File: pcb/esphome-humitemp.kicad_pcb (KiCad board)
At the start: 2 copper layers, 45 x 30 mm, 17 parts, among them J2 USB_IN, SW1 RESET, U1 SHT3x, U3 AMS1117-3.3, U4 ESP32-C3-MINI-1

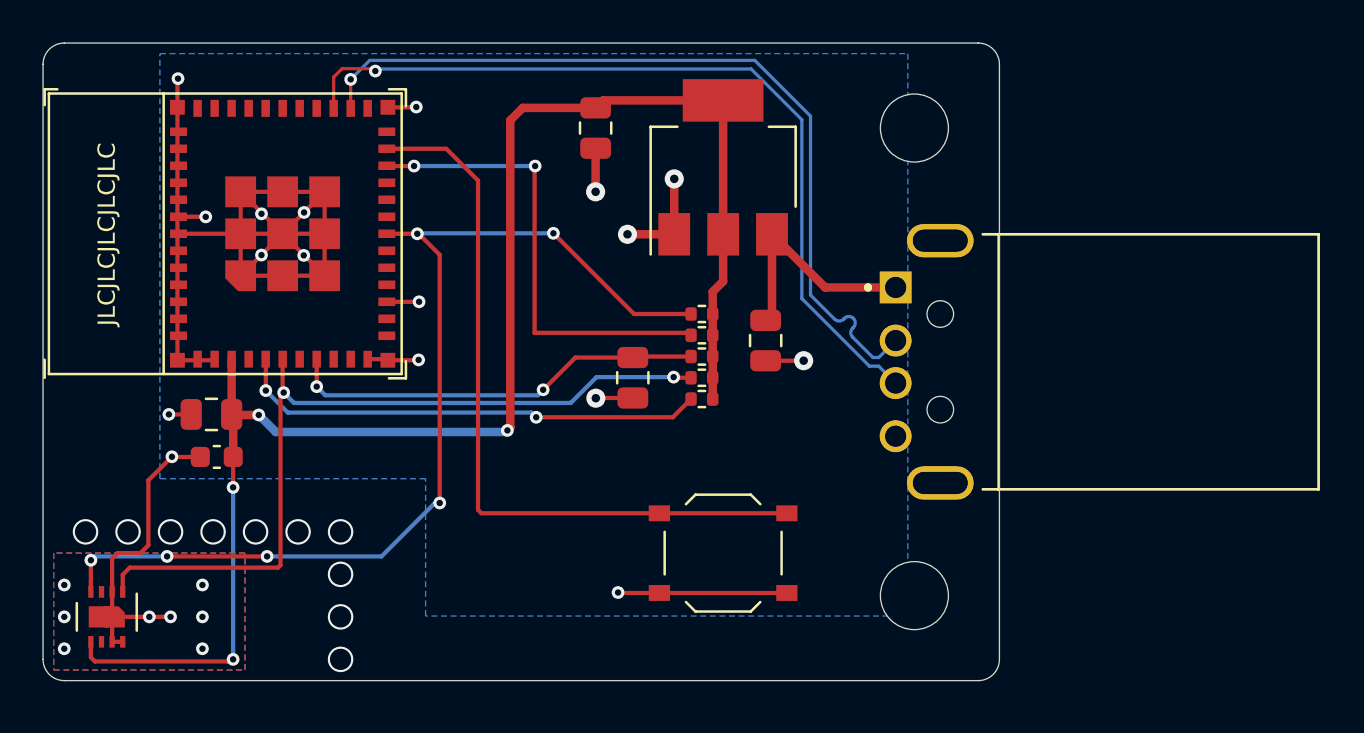
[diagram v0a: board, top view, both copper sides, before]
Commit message: rotate and send it
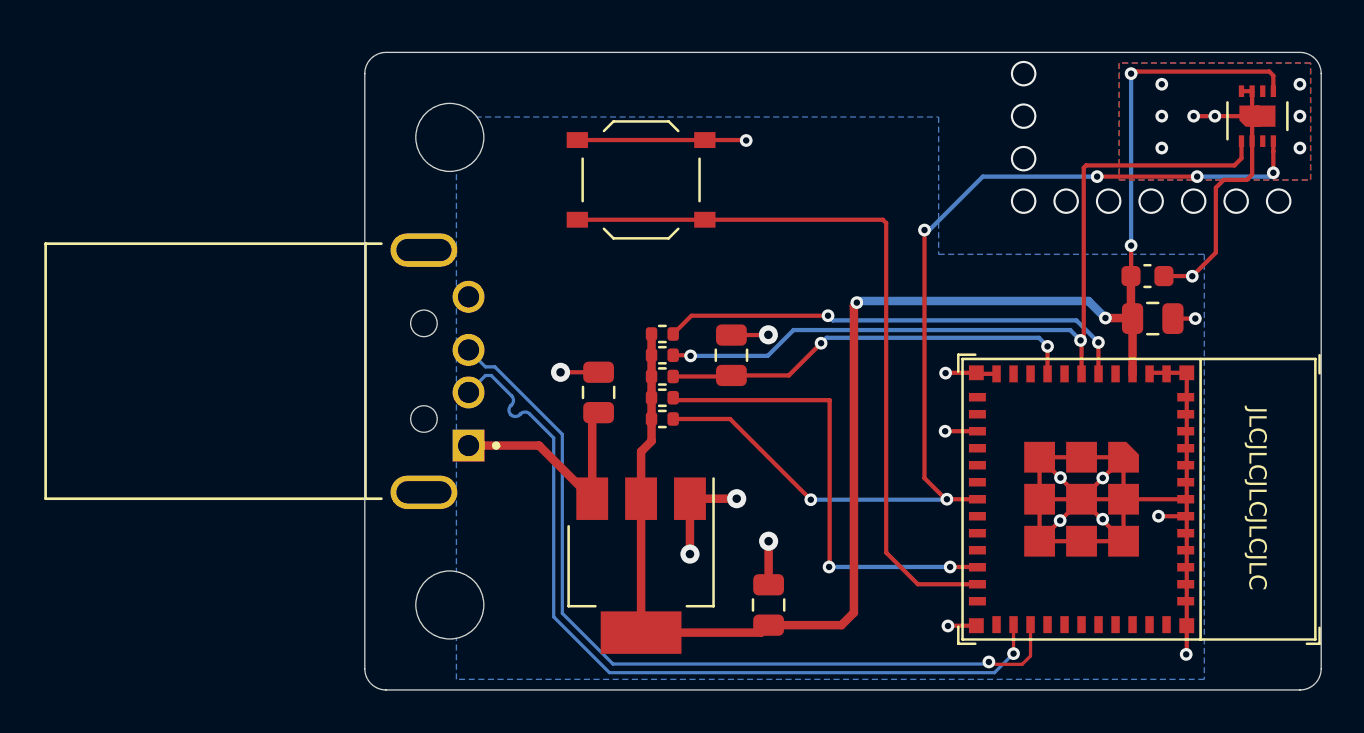
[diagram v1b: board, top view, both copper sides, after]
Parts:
- moved U1 59.0 mm to (147.1, 53.4), turned to 90 degrees
- moved U4 44.8 mm to (141.6, 71.5), turned to -90 degrees
- moved C5 44.6 mm to (142.0, 61.0), turned to 180 degrees
- moved C6 44.5 mm to (142.2, 63.0), turned to 180 degrees
- moved H1 31.3 mm to (109.1, 76.4), turned to 180 degrees
- moved H2 30.7 mm to (109.1, 54.4), turned to 180 degrees
- moved J2 24.3 mm to (107.9, 65.4), turned to -90 degrees
- moved C2 23.9 mm to (124.1, 76.4), turned to 90 degrees
- moved U3 19.1 mm to (118.1, 74.6), turned to -90 degrees
- moved SW1 18.0 mm to (118.1, 56.4), turned to 180 degrees
- moved C1 8.23 mm to (116.1, 66.4), turned to 90 degrees
- moved R3 5.28 mm to (119.1, 67.7), turned to 0 degrees
- moved C4 4.76 mm to (122.4, 64.7), turned to -90 degrees
- moved R5 3.58 mm to (119.1, 63.7), turned to 0 degrees
- moved R6 3.48 mm to (119.1, 66.7), turned to 0 degrees
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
